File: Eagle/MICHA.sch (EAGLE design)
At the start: 57 parts, among them IC1 LM4041A12LP, K1 PIN20X2, T1 BSS84, U1 ARDUINO_MKR_ZERO, U2 MIKROE_CLICK, X1 RJ45-RJULE4318101, X2 RJ45-RJULE4318101, X3 RJ45-RJULE4318101, X4 RJ45-RJULE4318101, X5 RJ45-RJULE4318101, X6 RJ45-RJULE4318101, X7 BUCHANAN_4_3.5MM

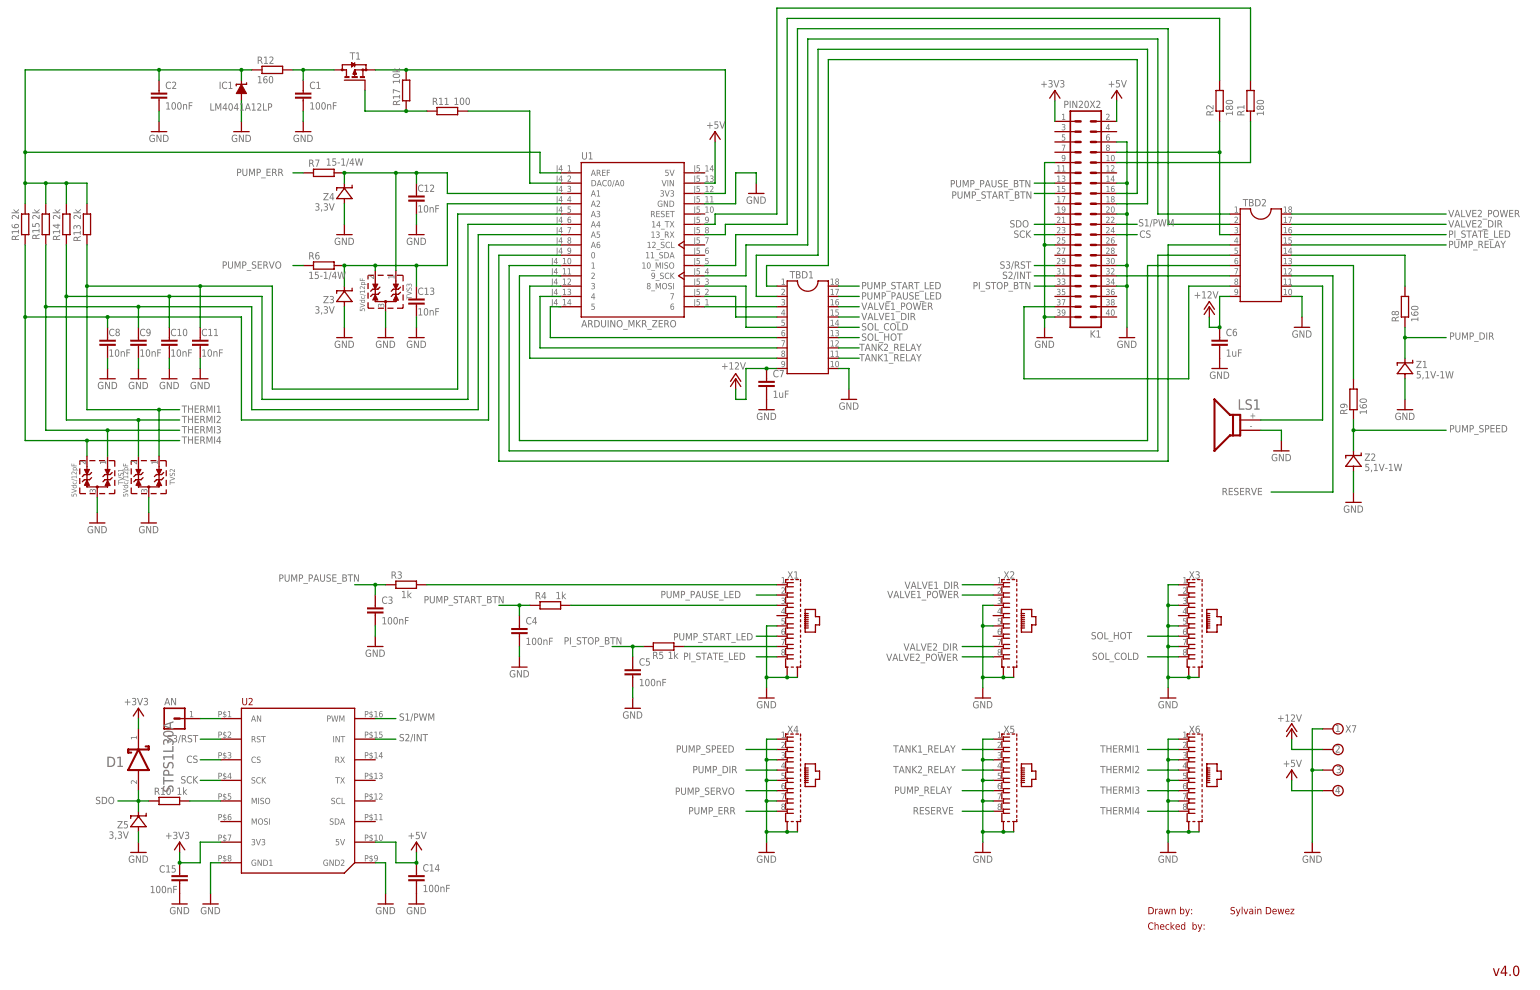
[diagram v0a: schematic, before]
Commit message: Downgrade to current version of PCB
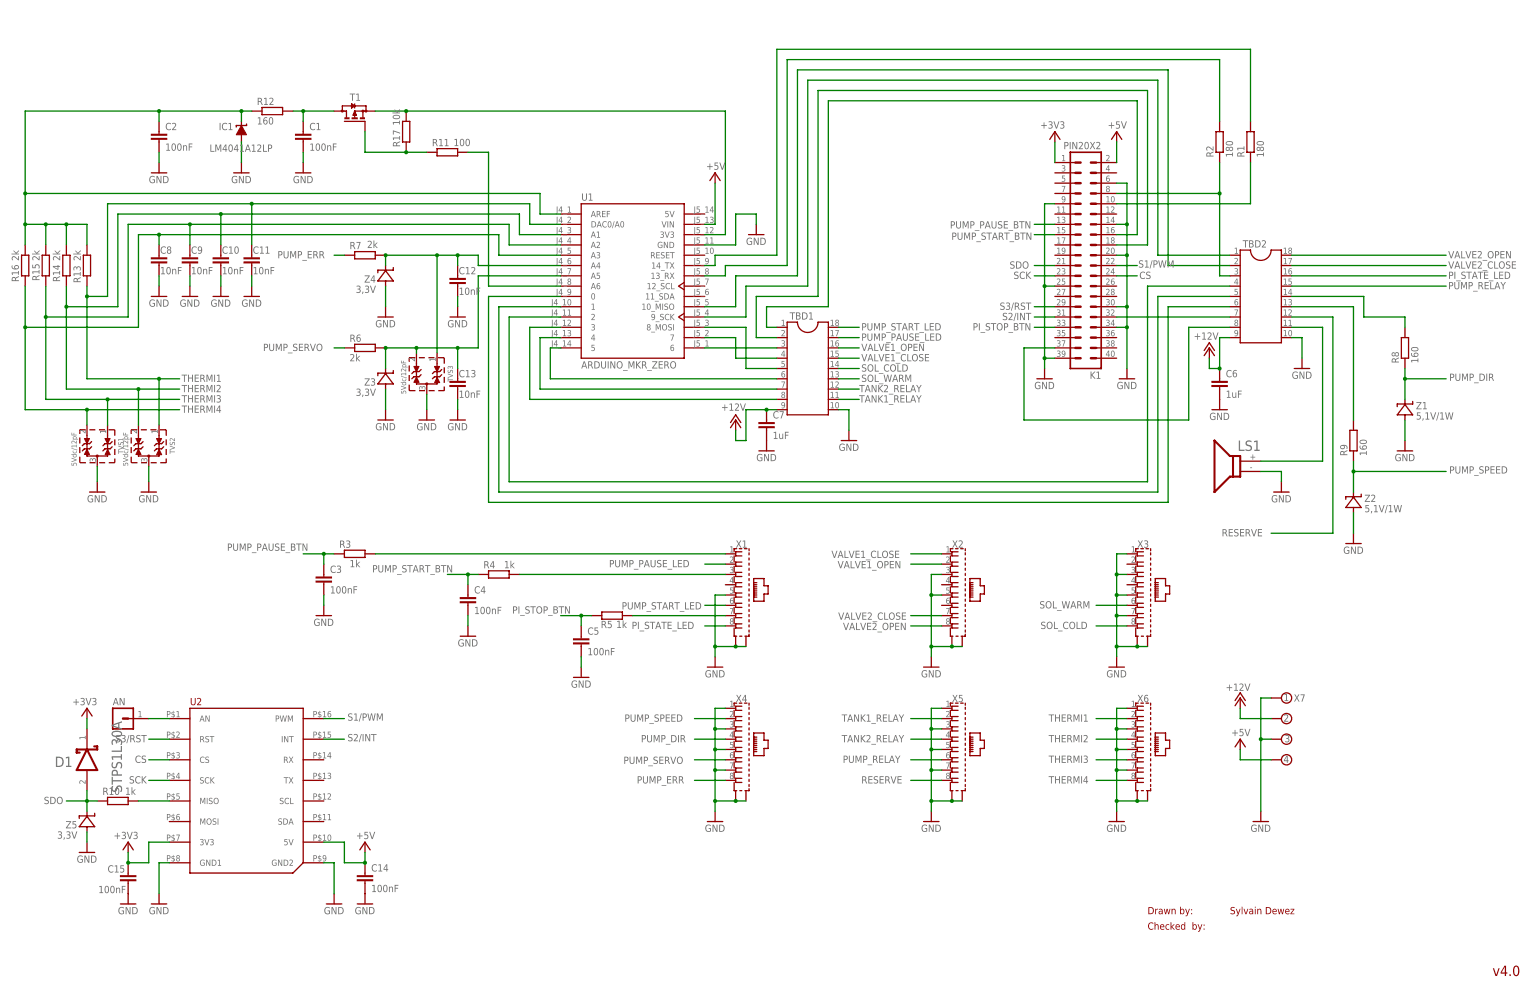
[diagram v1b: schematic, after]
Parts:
- R6, R7: value 15-1/4W -> 2k
- Z1, Z2: value 5,1V-1W -> 5,1V/1W
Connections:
- net SOL_HOT renamed SOL_WARM
- net VALVE1_DIR renamed VALVE1_CLOSE
- net VALVE1_POWER renamed VALVE1_OPEN
- net VALVE2_DIR renamed VALVE2_CLOSE
- net VALVE2_POWER renamed VALVE2_OPEN
- net D0: now also TBD2.6; no longer TBD2.4
- net D19: now also U1.A4; no longer U1.A1
- net D2: now also TBD2.4; no longer TBD2.6
- net D21: now also U1.A6; no longer U1.DAC0/A0
- net N$14: now also U1.A5; no longer U1.A2
- net THERMI1: now also U1.DAC0/A0; no longer U1.A3
- net THERMI2: now also U1.A1; no longer U1.A4
- net THERMI3: now also U1.A2; no longer U1.A5
- net THERMI4: now also U1.A3; no longer U1.A6
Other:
- moved on the sheet: AN, C1, C10, C11, C12, C13, C14, C15, C2, C3, C4, C5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
